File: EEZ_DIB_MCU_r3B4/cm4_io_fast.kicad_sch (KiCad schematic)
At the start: 1 part

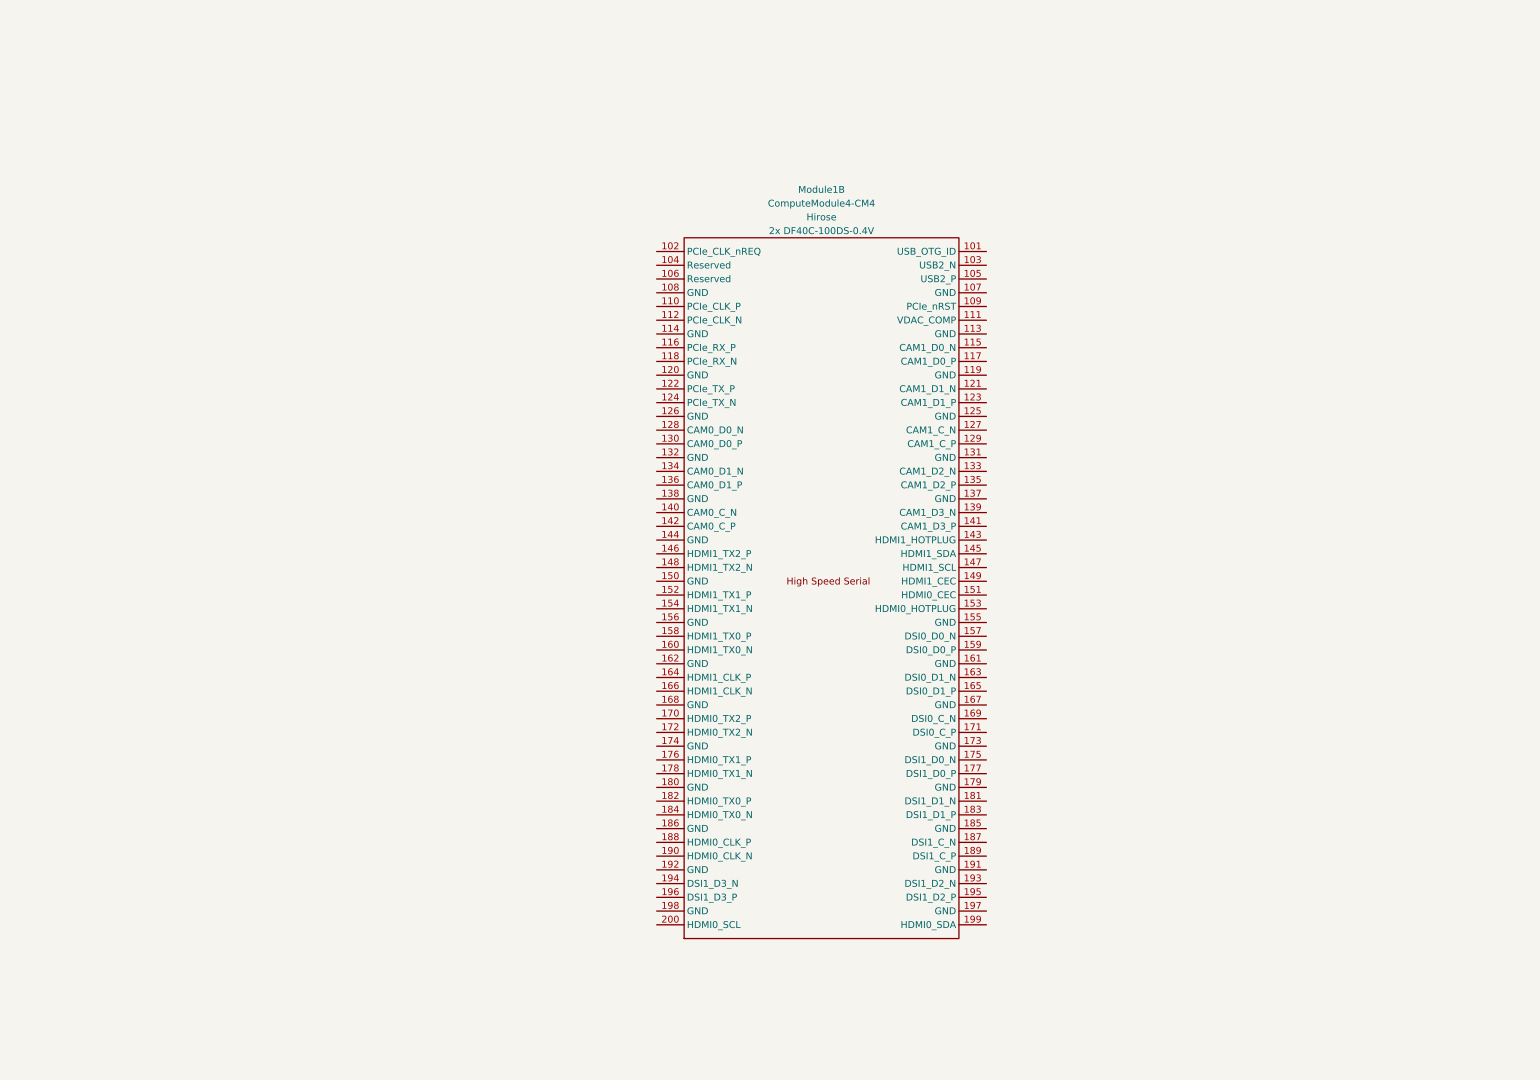
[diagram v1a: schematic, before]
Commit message: Adding ICN6211
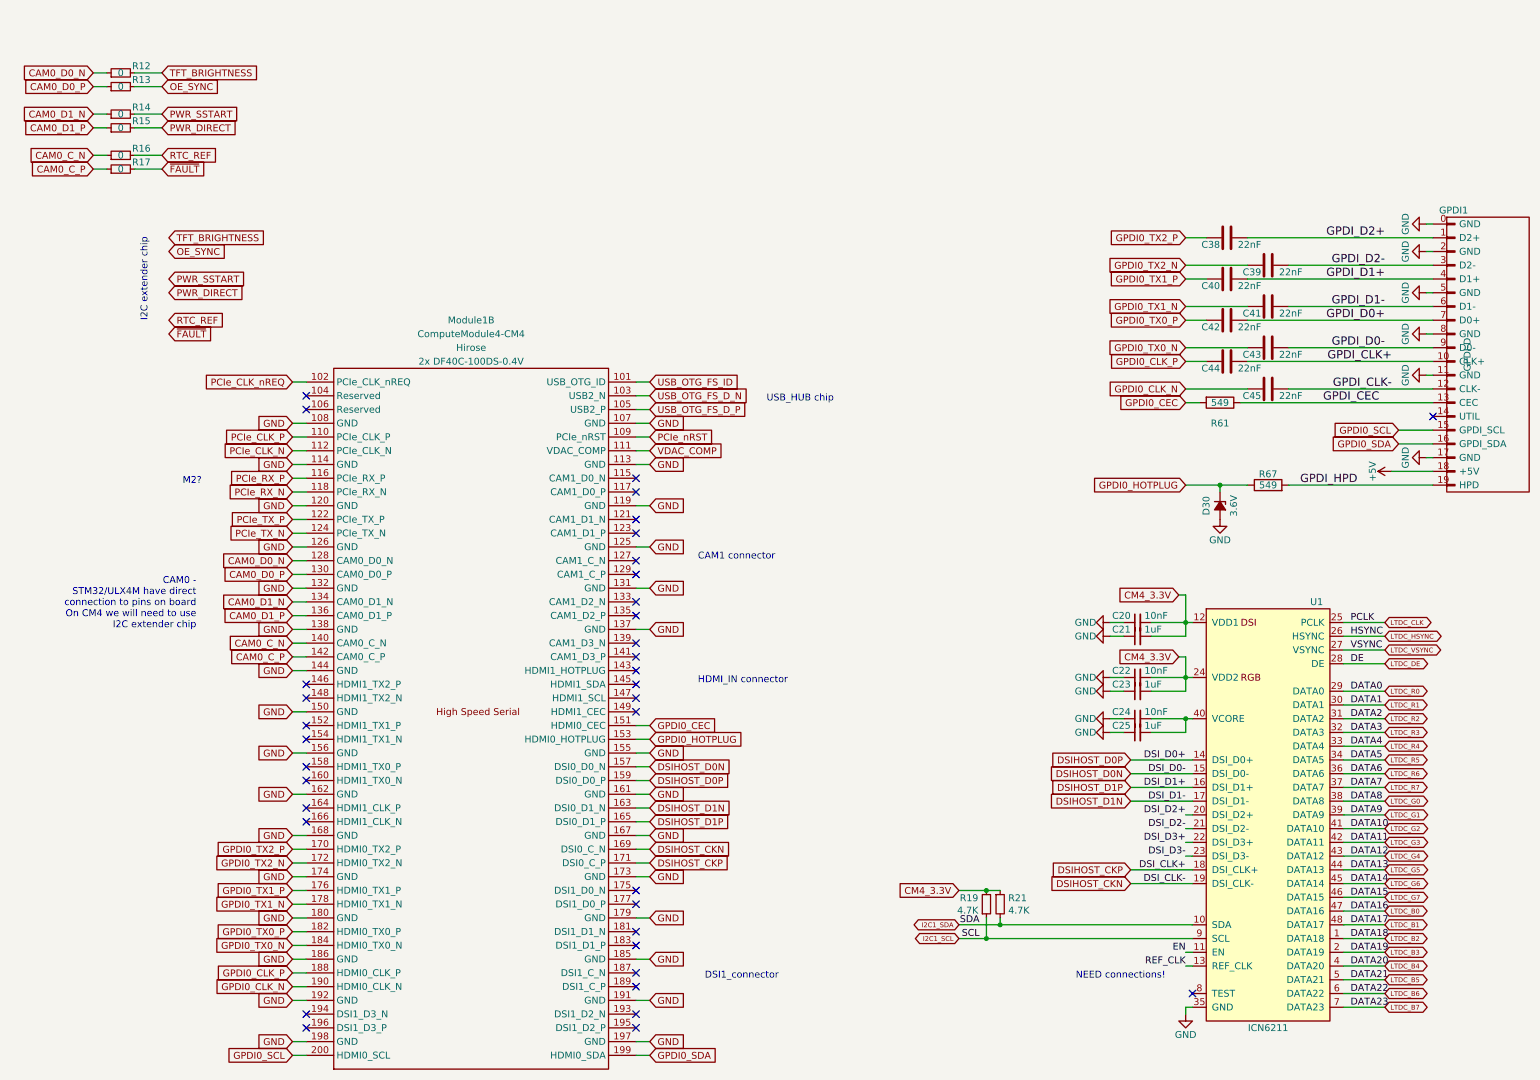
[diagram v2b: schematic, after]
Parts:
- added C20, C22, C24: 10nF, Capacitor_SMD:C_0603_1608Metric, symbol Device:C_Small
- added C21, C23, C25: 1uF, Capacitor_SMD:C_0603_1608Metric, symbol Device:C_Small
- added C38, C39, C40, C41, C42, C43, C44, C45: 22nF, Capacitor_SMD:C_0603_1608Metric, symbol Device:C
- added D30: 3.6V, Diode_SMD:D_SOD-323_HandSoldering, symbol ulx3s-rescue:D_Zener_Small_ALT-Device
- added GPDI1: GPDI-D, conn-fci:CONN-10029449-111RLF, symbol hdmi-d:HDMI-D
- added R12, R13, R14, R15, R16, R17: 0, Resistor_SMD:R_0603_1608Metric, symbol Device:R_Small
- added R19, R21: 4.7K, Resistor_SMD:R_0603_1608Metric, symbol Device:R_Small
- added R61, R67: 549, Resistor_SMD:R_0603_1608Metric, symbol Device:R
- added U1: ICN6211, Package_DFN_QFN:QFN-48-1EP_6x6mm_P0.4mm_EP4.2x4.2mm, symbol ICN6211_breakout-rescue:ICN6211-Interface_Display_Extra
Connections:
- net USB_OTG_FS_ID: now reaches Module1.101 (USB_OTG_ID)
- net PCIe_CLK_nREQ: now reaches Module1.102 (PCIe_CLK_nREQ)
- net USB_OTG_FS_D_N: now reaches Module1.103 (USB2_N)
- net USB_OTG_FS_D_P: now reaches Module1.105 (USB2_P)
- net GND: now reaches Module1.107 (GND)
- net GND: now also Module1.108 (GND), Module1.113 (GND), Module1.114 (GND), Module1.119 (GND), Module1.120 (GND), Module1.125 (GND), Module1.126 (GND), Module1.131 (GND), Module1.132 (GND), Module1.137 (GND), Module1.138 (GND), Module1.144 (GND), Module1.150 (GND), Module1.155 (GND), Module1.156 (GND), Module1.161 (GND), Module1.162 (GND), Module1.167 (GND), Module1.168 (GND), Module1.173 (GND), Module1.174 (GND), Module1.179 (GND), Module1.180 (GND), Module1.185 (GND), Module1.186 (GND), Module1.191 (GND), Module1.192 (GND), Module1.197 (GND), Module1.198 (GND), C20.1, C21.1, C22.1, C23.1, C24.1, C25.1, D30.2 (A), GPDI1.0 (GND), GPDI1.11 (GND), GPDI1.17 (GND), GPDI1.2 (GND), GPDI1.5 (GND), GPDI1.8 (GND), U1.35 (GND), U1.49 (PAD)
- net PCIe_nRST: now reaches Module1.109 (PCIe_nRST)
- net PCIe_CLK_P: now reaches Module1.110 (PCIe_CLK_P)
- net VDAC_COMP: now reaches Module1.111 (VDAC_COMP)
- net PCIe_CLK_N: now reaches Module1.112 (PCIe_CLK_N)
- net PCIe_RX_P: now reaches Module1.116 (PCIe_RX_P)
- net PCIe_RX_N: now reaches Module1.118 (PCIe_RX_N)
- net PCIe_TX_P: now reaches Module1.122 (PCIe_TX_P)
- net PCIe_TX_N: now reaches Module1.124 (PCIe_TX_N)
- net CAM0_D0_N: now reaches Module1.128 (CAM0_D0_N)
- net CAM0_D0_N: now also R12.1
- net CAM0_D0_P: now reaches Module1.130 (CAM0_D0_P)
- net CAM0_D0_P: now also R13.1
- net CAM0_D1_N: now reaches Module1.134 (CAM0_D1_N)
- net CAM0_D1_N: now also R14.1
- net CAM0_D1_P: now reaches Module1.136 (CAM0_D1_P)
- net CAM0_D1_P: now also R15.1
- net CAM0_C_N: now reaches Module1.140 (CAM0_C_N)
- net CAM0_C_N: now also R16.1
- net CAM0_C_P: now reaches Module1.142 (CAM0_C_P)
- net CAM0_C_P: now also R17.1
- net GPDI0_CEC: now reaches Module1.151 (HDMI0_CEC)
- net GPDI0_CEC: now also R61.2
- net GPDI0_HOTPLUG: now reaches Module1.153 (HDMI0_HOTPLUG)
- net GPDI0_HOTPLUG: now also D30.1 (K), R67.1
- net DSIHOST_D0N: now reaches Module1.157 (DSI0_D0_N)
- net DSIHOST_D0N: now also U1.15 (DSI_D0-)
- net DSIHOST_D0P: now reaches Module1.159 (DSI0_D0_P)
- net DSIHOST_D0P: now also U1.14 (DSI_D0+)
- net DSIHOST_D1N: now reaches Module1.163 (DSI0_D1_N)
- net DSIHOST_D1N: now also U1.17 (DSI_D1-)
- net DSIHOST_D1P: now reaches Module1.165 (DSI0_D1_P)
- net DSIHOST_D1P: now also U1.16 (DSI_D1+)
- net DSIHOST_CKN: now reaches Module1.169 (DSI0_C_N)
- net DSIHOST_CKN: now also U1.19 (DSI_CLK-)
- net GPDI0_TX2_P: now reaches Module1.170 (HDMI0_TX2_P)
- net GPDI0_TX2_P: now also C38.1
- net DSIHOST_CKP: now reaches Module1.171 (DSI0_C_P)
- net DSIHOST_CKP: now also U1.18 (DSI_CLK+)
- net GPDI0_TX2_N: now reaches Module1.172 (HDMI0_TX2_N)
- net GPDI0_TX2_N: now also C39.1
- net GPDI0_TX1_P: now reaches Module1.176 (HDMI0_TX1_P)
- net GPDI0_TX1_P: now also C40.1
- net GPDI0_TX1_N: now reaches Module1.178 (HDMI0_TX1_N)
- net GPDI0_TX1_N: now also C41.1
- net GPDI0_TX0_P: now reaches Module1.182 (HDMI0_TX0_P)
- net GPDI0_TX0_P: now also C42.1
- net GPDI0_TX0_N: now reaches Module1.184 (HDMI0_TX0_N)
- net GPDI0_TX0_N: now also C43.1
- net GPDI0_CLK_P: now reaches Module1.188 (HDMI0_CLK_P)
- net GPDI0_CLK_P: now also C44.1
- net GPDI0_CLK_N: now reaches Module1.190 (HDMI0_CLK_N)
- net GPDI0_CLK_N: now also C45.1
- net GPDI0_SDA: now reaches Module1.199 (HDMI0_SDA)
- net GPDI0_SDA: now also GPDI1.16 (GPDI_SDA)
- net GPDI0_SCL: now reaches Module1.200 (HDMI0_SCL)
- net GPDI0_SCL: now also GPDI1.15 (GPDI_SCL)
- new net: C24.2, C25.2, U1.40 (VCORE)
- new net +5V: GPDI1.18 (+5V)
- new net CM4_3.3V: C20.2, C21.2, C22.2, C23.2, R19.2, R21.1, U1.12 (VDD1), U1.24 (VDD2), U1.3 (VDD3)
- new net DSI_D2+: U1.20 (DSI_D2+)
- new net DSI_D2-: U1.21 (DSI_D2-)
- new net DSI_D3+: U1.22 (DSI_D3+)
- new net DSI_D3-: U1.23 (DSI_D3-)
- new net EN: U1.11 (EN)
- new net GPDI_CEC: GPDI1.13 (CEC), R61.1
- new net GPDI_CLK+: C44.2, GPDI1.10 (CLK+)
- new net GPDI_CLK-: C45.2, GPDI1.12 (CLK-)
- new net GPDI_D0+: C42.2, GPDI1.7 (D0+)
- new net GPDI_D0-: C43.2, GPDI1.9 (D0-)
- new net GPDI_D1+: C40.2, GPDI1.4 (D1+)
- new net GPDI_D1-: C41.2, GPDI1.6 (D1-)
- new net GPDI_D2+: C38.2, GPDI1.1 (D2+)
- new net GPDI_D2-: C39.2, GPDI1.3 (D2-)
- new net GPDI_HPD: GPDI1.19 (HPD), R67.2
- new net I2C1_SCL: R19.1, U1.9 (SCL)
- new net I2C1_SDA: R21.2, U1.10 (SDA)
- new net LTDC_B0: U1.47 (DATA16)
- new net LTDC_B1: U1.48 (DATA17)
- new net LTDC_B2: U1.1 (DATA18)
- new net LTDC_B3: U1.2 (DATA19)
- new net LTDC_B4: U1.4 (DATA20)
- new net LTDC_B5: U1.5 (DATA21)
- new net LTDC_B6: U1.6 (DATA22)
- new net LTDC_B7: U1.7 (DATA23)
- new net LTDC_CLK: U1.25 (PCLK)
- new net LTDC_DE: U1.28 (DE)
- new net LTDC_G0: U1.38 (DATA8)
- new net LTDC_G1: U1.39 (DATA9)
- new net LTDC_G2: U1.41 (DATA10)
- new net LTDC_G3: U1.42 (DATA11)
- new net LTDC_G4: U1.43 (DATA12)
- new net LTDC_G5: U1.44 (DATA13)
- new net LTDC_G6: U1.45 (DATA14)
- new net LTDC_G7: U1.46 (DATA15)
- new net LTDC_HSYNC: U1.26 (HSYNC)
- new net LTDC_R0: U1.29 (DATA0)
- new net LTDC_R1: U1.30 (DATA1)
- new net LTDC_R2: U1.31 (DATA2)
- new net LTDC_R3: U1.32 (DATA3)
- new net LTDC_R4: U1.33 (DATA4)
- new net LTDC_R5: U1.34 (DATA5)
- new net LTDC_R6: U1.36 (DATA6)
- new net LTDC_R7: U1.37 (DATA7)
- new net LTDC_VSYNC: U1.27 (VSYNC)
- new net OE_SYNC: R13.2
- new net PWR_DIRECT: R15.2
- new net PWR_SSTART: R14.2
- new net REF_CLK: U1.13 (REF_CLK)
- new net RTC_REF: R16.2
- new net TFT_BRIGHTNESS: R12.2
- new net ~{FAULT}: R17.2
- no-connect marks 0 -> 36
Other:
- note added: "CAM0 - STM32/ULX4M have direct connection to pins on board On CM4 we will need to use I2C extender chip"
- note added: "CAM1 connector"
- note added: "DSI1_connector"
- note added: "HDMI_IN connector"
- note added: "I2C extender chip"
- note added: "M2?"
- note added: "NEED connections!"
- note added: "USB_HUB chip"
- moved on the sheet: Module1B

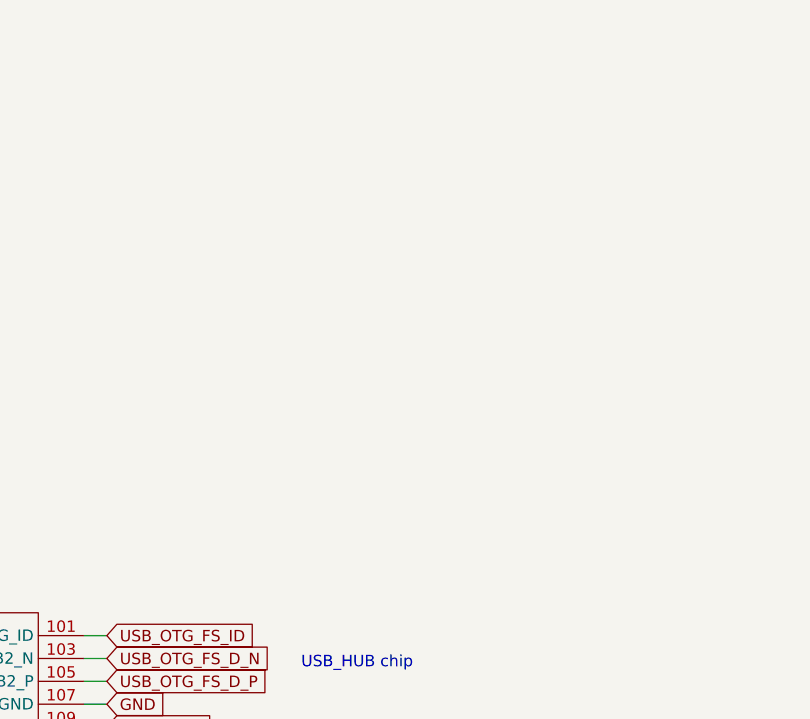
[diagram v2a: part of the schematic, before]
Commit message: Adding DSI connector
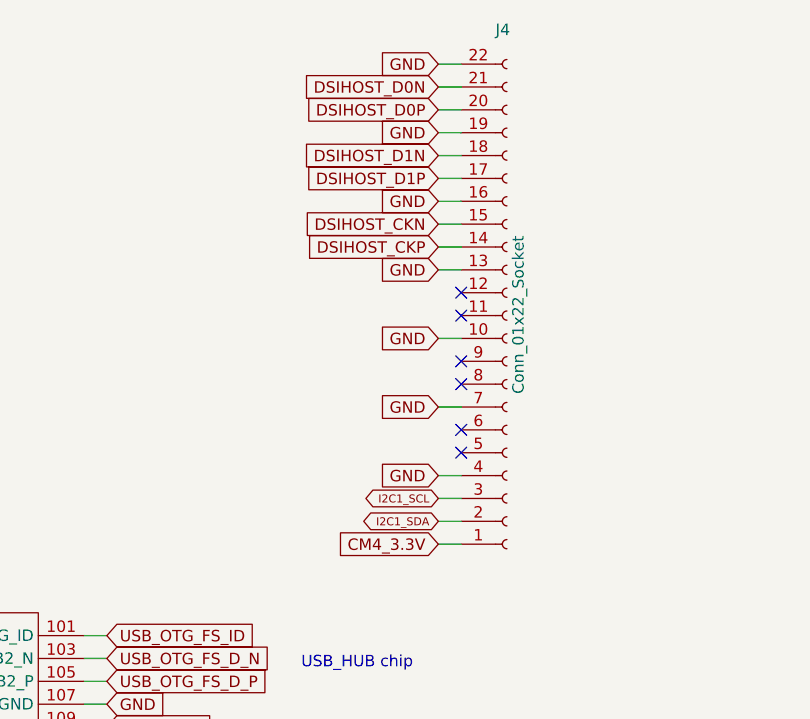
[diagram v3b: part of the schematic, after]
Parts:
- added J4: Conn_01x22_Socket, Connector_FFC-FPC:Hirose_FH12-22S-0.5SH_1x22-1MP_P0.50mm_Horizontal, symbol Connector:Conn_01x22_Socket
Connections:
- net CM4_3.3V: now also J4.1 (Pin_1)
- net DSIHOST_CKN: now also J4.15 (Pin_15)
- net DSIHOST_CKP: now also J4.14 (Pin_14)
- net DSIHOST_D0N: now also J4.21 (Pin_21)
- net DSIHOST_D0P: now also J4.20 (Pin_20)
- net DSIHOST_D1N: now also J4.18 (Pin_18)
- net DSIHOST_D1P: now also J4.17 (Pin_17)
- net GND: now also J4.10 (Pin_10), J4.13 (Pin_13), J4.16 (Pin_16), J4.19 (Pin_19), J4.22 (Pin_22), J4.4 (Pin_4), J4.7 (Pin_7)
- net I2C1_SCL: now also J4.3 (Pin_3)
- net I2C1_SDA: now also J4.2 (Pin_2)
- no-connect marks 36 -> 42

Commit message: Updating License informations
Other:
- company: (none) -> Intergalaktik d.o.o.
- title: (none) -> BB3 CM3
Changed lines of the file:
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@@
 (kicad_sch (version 20230121) (generator eeschema)
   (paper "A4")
+  (title_block
+    (title "BB3 CM3")
+    (date "2023-06-28")
+    (rev "v001")
+    (company "Intergalaktik d.o.o.")
+    (comment 1 "This hardware is licensed under CERN-OHL-S v2 or later.")
+  )
   (junction (at 186.69 165.1) (diameter 0) (color 0 0 0 0)
   )
